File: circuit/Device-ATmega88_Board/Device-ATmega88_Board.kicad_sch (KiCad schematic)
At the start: 24 parts, among them J1 7seg, J2 USB_A, J3 Conn_01x06_Female, J4 Conn_01x06_Female, J5 ICSP, Q1 2SC1815, Q2 2SC1815, Q3 2SC1815, Q4 2SC1815, U1 ATmega328P-P

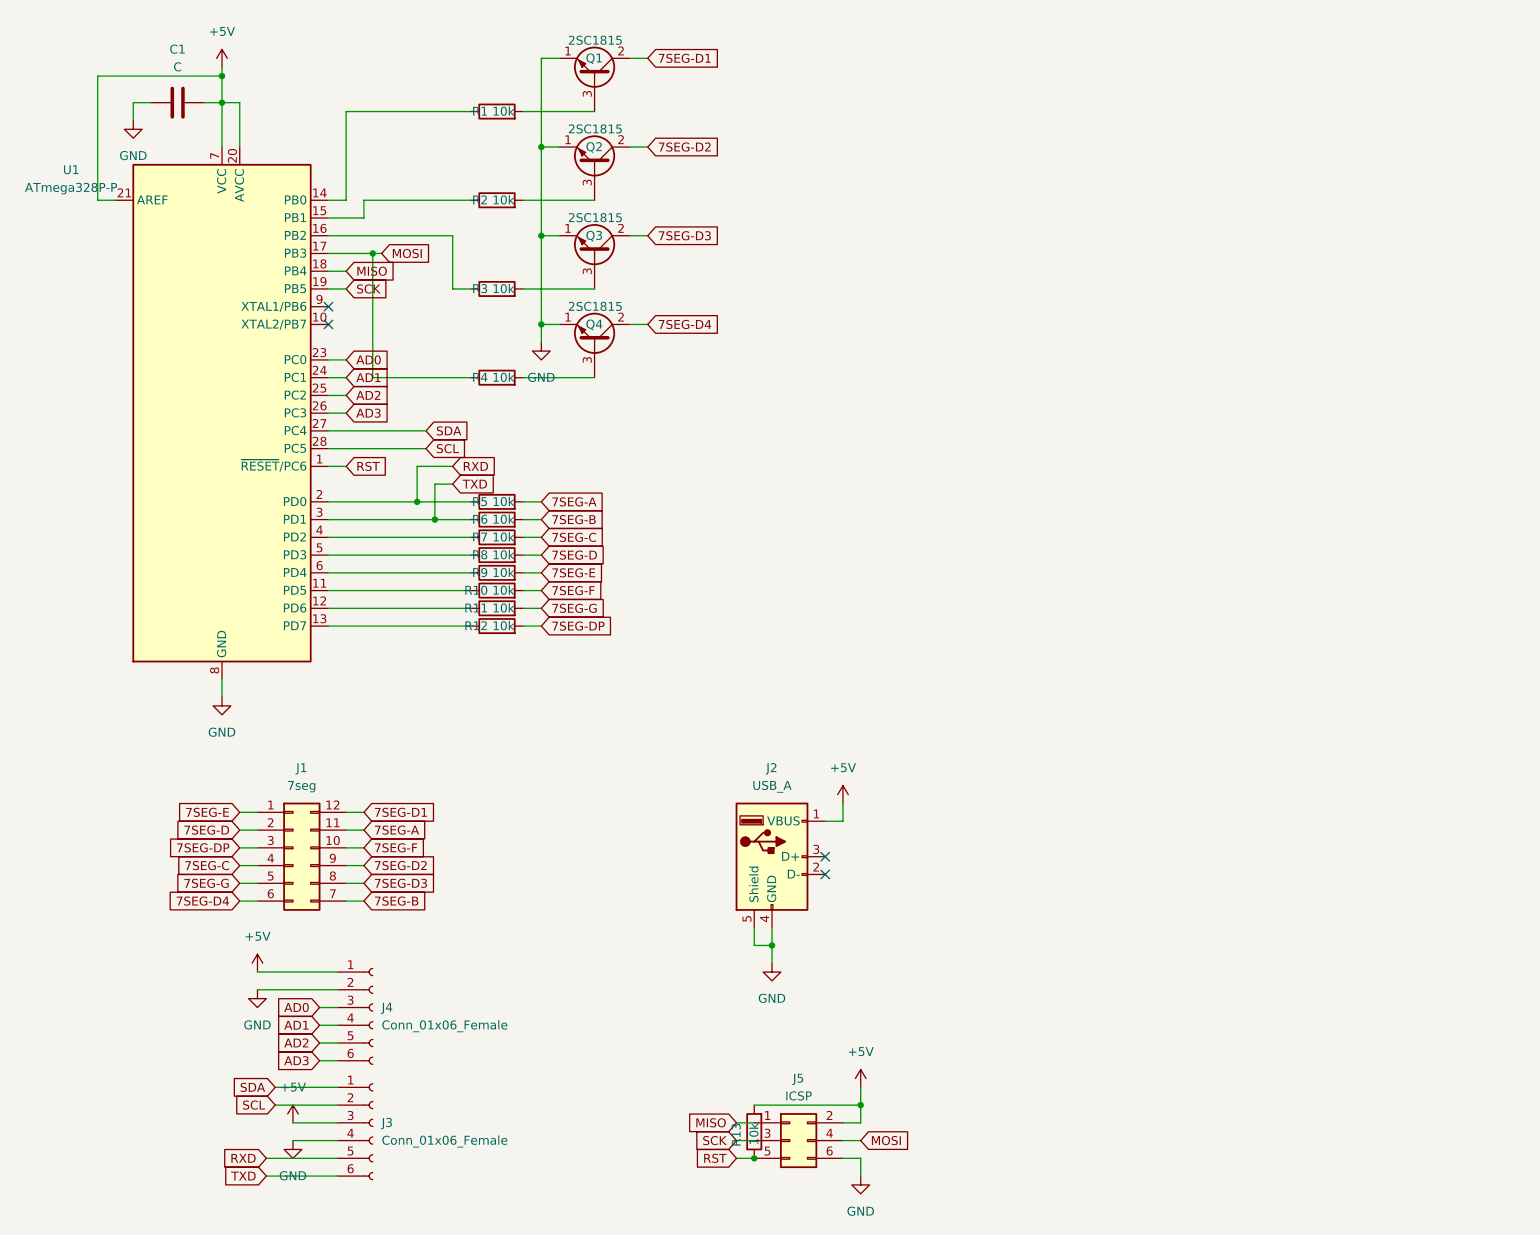
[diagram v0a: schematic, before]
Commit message: プログラムを追加
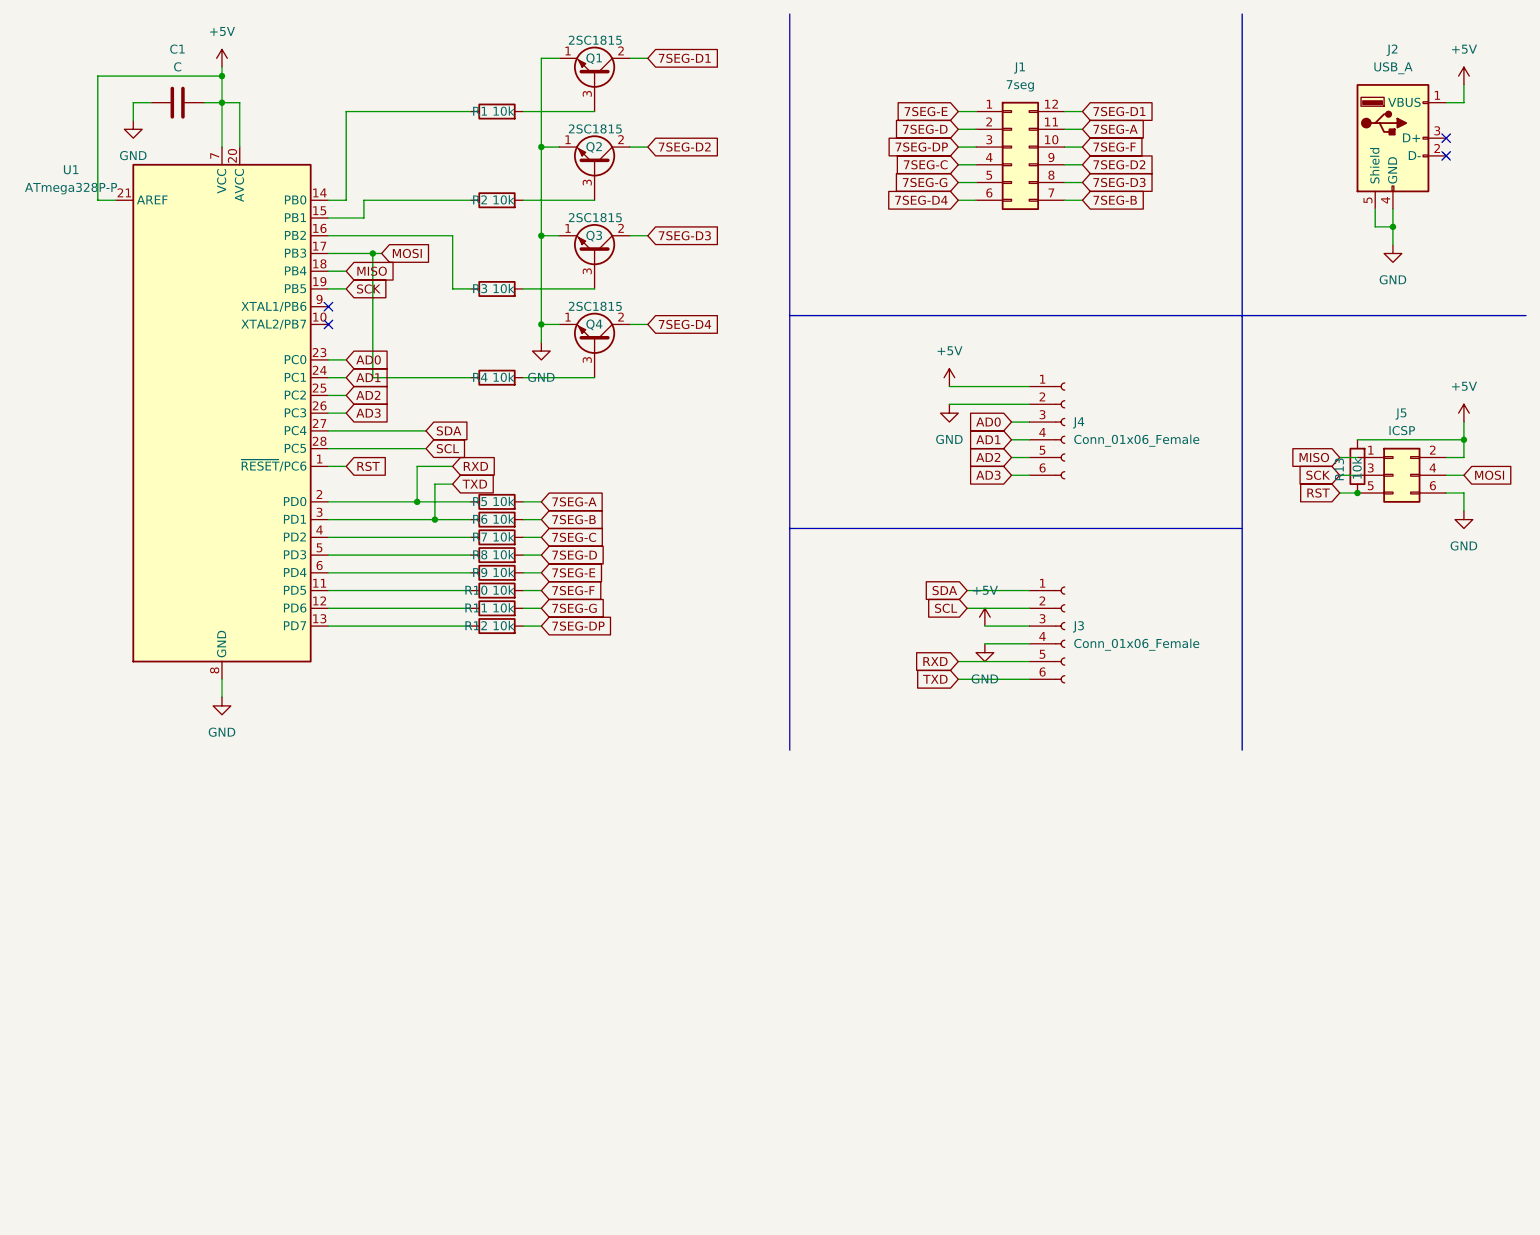
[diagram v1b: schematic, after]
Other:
- moved on the sheet: J1, J2, J3, J4, J5, R13
